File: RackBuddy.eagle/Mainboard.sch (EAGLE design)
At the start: 12 parts, among them IC1 ATmega328, Q1 16MHz, Q2 BC337-40

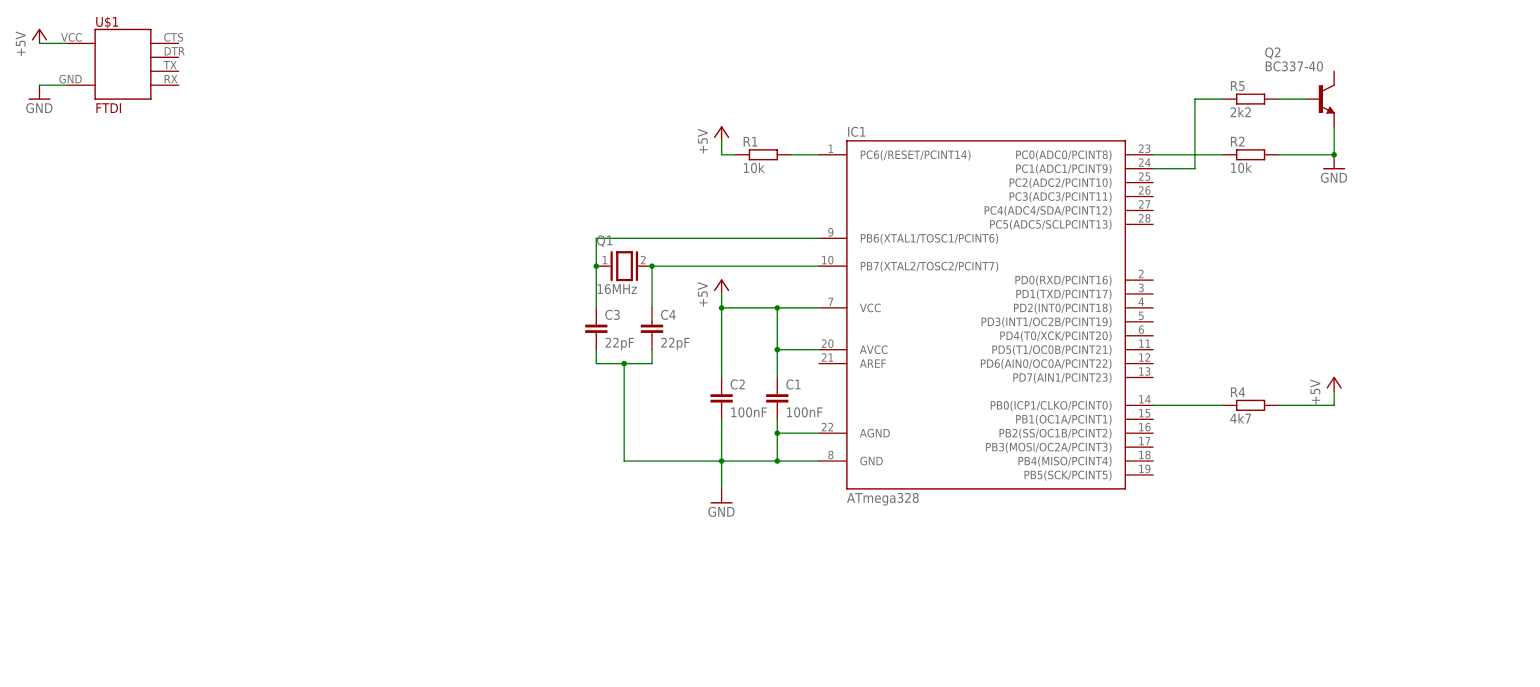
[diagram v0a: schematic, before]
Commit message: An den Plänen gearbeitet
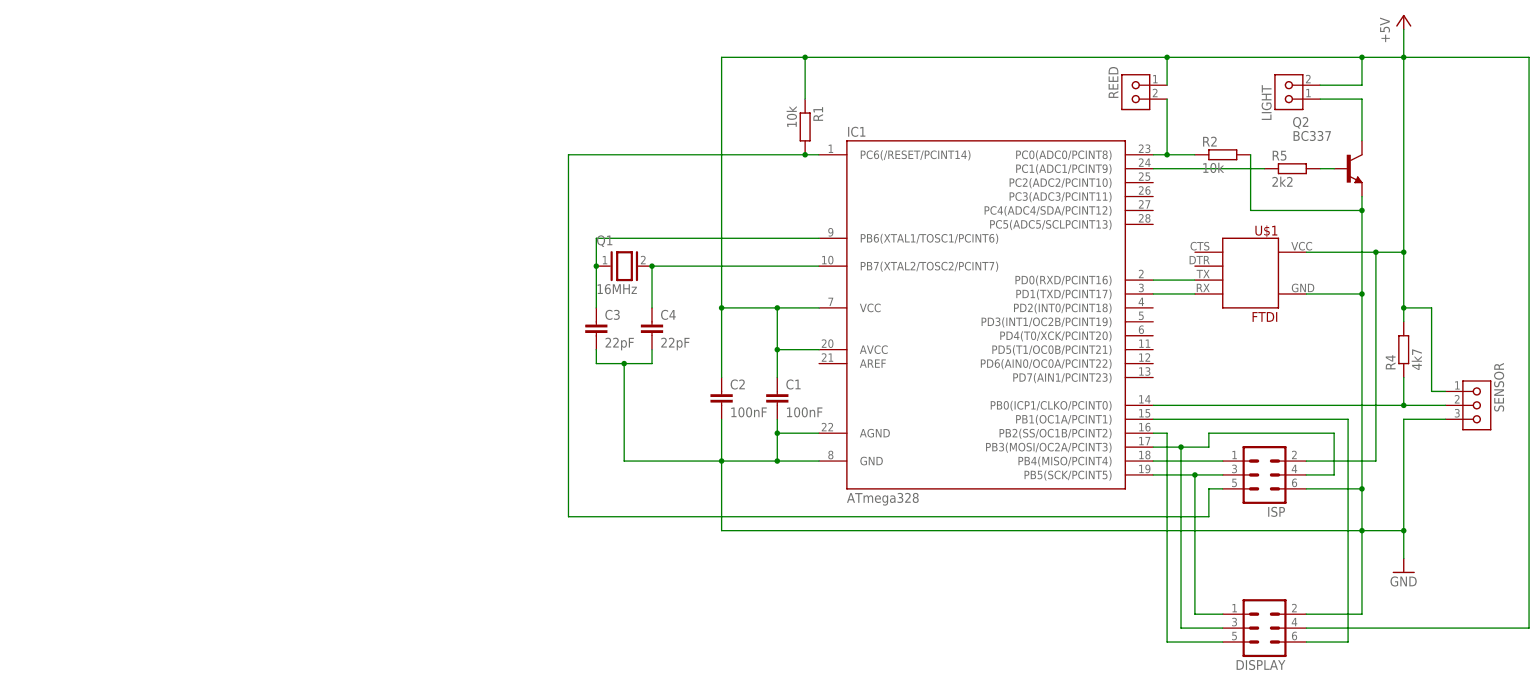
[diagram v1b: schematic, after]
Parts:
- added DISPLAY, ISP: (no value), con-ml:ML6
- added LIGHT, REED: KK2VSQ, molex-kk:KK2VSQ
- added SENSOR: KK3V, molex-kk:KK3V
- Q2: value BC337-40 -> BC337; device transistor-npn:BC337-40 -> Zap-Verbogene Teile:BC337
- R1: device rcl:R-EU_0204/7 -> rcl:R-EU_0207/10
- R2: device rcl:R-EU_0204/7 -> rcl:R-EU_0204/2V
- U$1: device USB-Breakouts:FTDI -> Zap-USB-Breakouts:FTDI
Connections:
- new net N$11: LIGHT.1, Q2.C
- new net N$12: DISPLAY.5, IC1.PB2(SS/OC1B/PCINT2)
- new net N$13: IC1.PB4(MISO/PCINT4), ISP.1
- new net N$14: DISPLAY.1, IC1.PB5(SCK/PCINT5), ISP.3
- new net N$16: DISPLAY.6, IC1.PB1(OC1A/PCINT1)
- new net N$3: IC1.PD0(RXD/PCINT16), U$1.TX
- new net N$4: IC1.PD1(TXD/PCINT17), U$1.RX
- new net N$7: DISPLAY.3, IC1.PB3(MOSI/OC2A/PCINT3), ISP.4
- net +5V: now also DISPLAY.4, ISP.2, LIGHT.2, REED.1, SENSOR.1
- net GND: now also DISPLAY.2, ISP.6, SENSOR.3
- net N$10: now also SENSOR.2
- net N$8: now also ISP.5
- net N$9: now also REED.2
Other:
- moved on the sheet: Q2, R1, R2, R4, R5, U$1
